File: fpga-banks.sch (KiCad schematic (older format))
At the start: 3 parts, among them U1 XC7K70T-FBG484, U2 ASEM1-100.000MHZ-LC-T

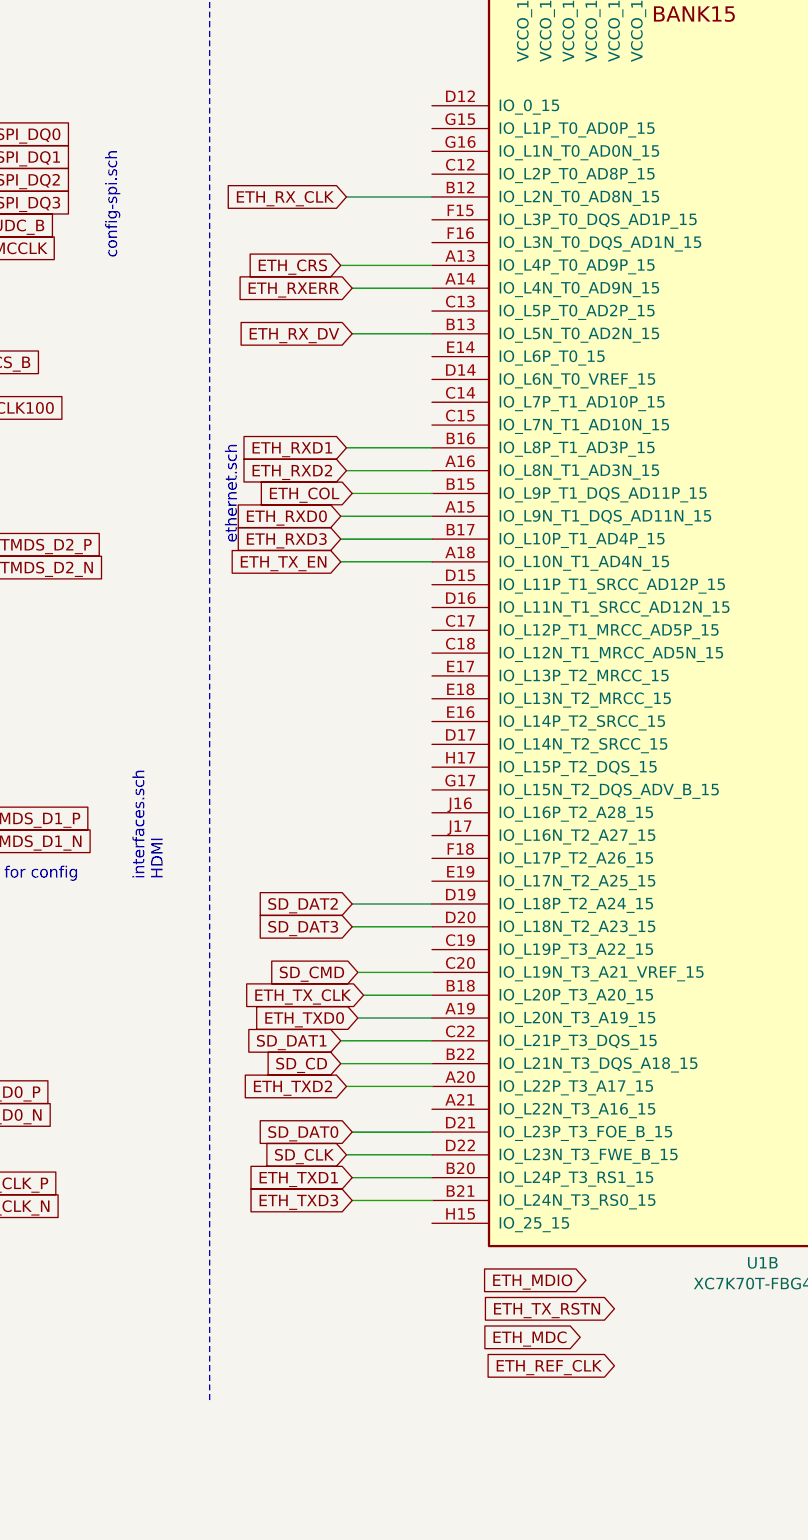
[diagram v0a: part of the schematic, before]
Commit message: Connected RGMII - Wip
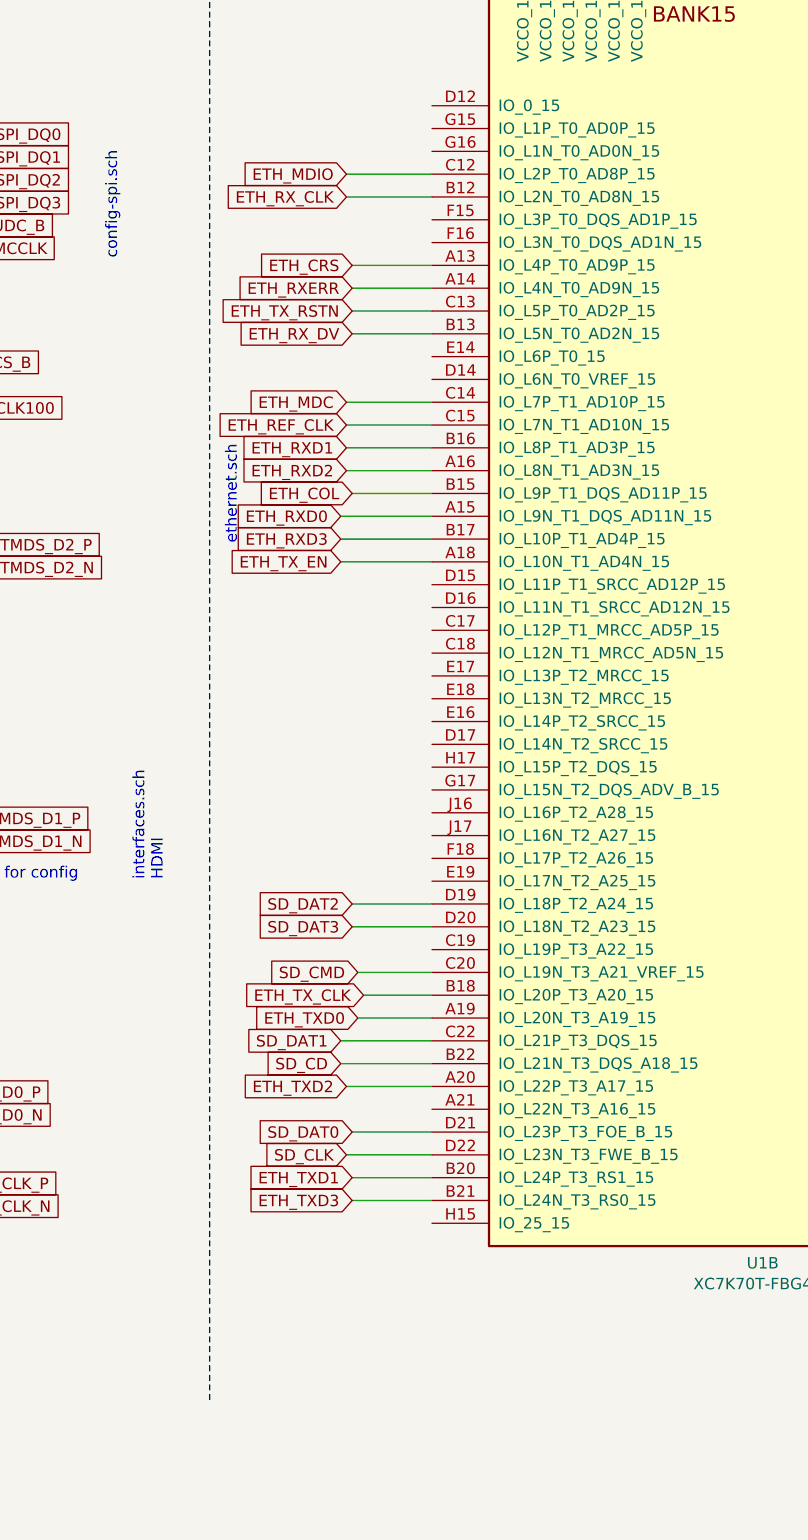
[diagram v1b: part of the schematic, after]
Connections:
- net ETH_MDC: now also U1.C14 (IO_L7P_T1_AD10P_15)
- net ETH_MDIO: now also U1.C12 (IO_L2P_T0_AD8P_15)
- net ETH_REF_CLK: now also U1.C15 (IO_L7N_T1_AD10N_15)
- net ETH_TX_RSTN: now also U1.C13 (IO_L5P_T0_AD2P_15)
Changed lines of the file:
@@
 	8400 1350 8400 1250
 Connection ~ 8225 1350
-Text GLabel 8125 7800 0    50   Input ~ 0
-ETH_REF_CLK
 Text GLabel 6925 4075 0    50   Input ~ 0
 ETH_RXD0
@@
 Text GLabel 6975 3075 0    50   Input ~ 0
 ETH_RXERR
-Text GLabel 8125 7550 0    50   Input ~ 0
+Text GLabel 6975 3175 0    50   Input ~ 0
 ETH_TX_RSTN
 Text GLabel 6925 4275 0    50   Input ~ 0
@@
 Text GLabel 6950 6575 0    50   Input ~ 0
 ETH_TXD2
-Text GLabel 8000 7425 0    50   Input ~ 0
+Text GLabel 6950 2575 0    50   Input ~ 0
 ETH_MDIO
 Text GLabel 6975 3975 0    50   Input ~ 0
@@
 Text GLabel 6950 3775 0    50   Input ~ 0
 ETH_RXD1
-Text GLabel 6925 2975 0    50   Input ~ 0
+Text GLabel 6975 2975 0    50   Input ~ 0
 ETH_CRS
 Text GLabel 7000 6275 0    50   Input ~ 0
 ETH_TXD0
-Text GLabel 7975 7675 0    50   Input ~ 0
+Text GLabel 6950 3575 0    50   Input ~ 0
 ETH_MDC
 Text GLabel 6950 2675 0    50   Input ~ 0
@@
 	6975 3275 7325 3275
 Wire Wire Line
-	6925 2975 7325 2975
+	6975 2975 7325 2975
 Wire Wire Line
 	6925 4075 7325 4075
@@
 Wire Wire Line
 	12100 3025 11825 3025
+Wire Wire Line
+	7325 2575 6950 2575
+Wire Wire Line
+	7325 3175 6975 3175
+Wire Wire Line
+	7325 3575 6950 3575
+Wire Wire Line
+	7325 3675 6950 3675
+Text GLabel 6950 3675 0    50   Input ~ 0
+ETH_REF_CLK
 $EndSCHEMATC
